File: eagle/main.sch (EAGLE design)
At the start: 43 parts, among them Q1 SQJ886EP, U1 LTC3789EGNPBF

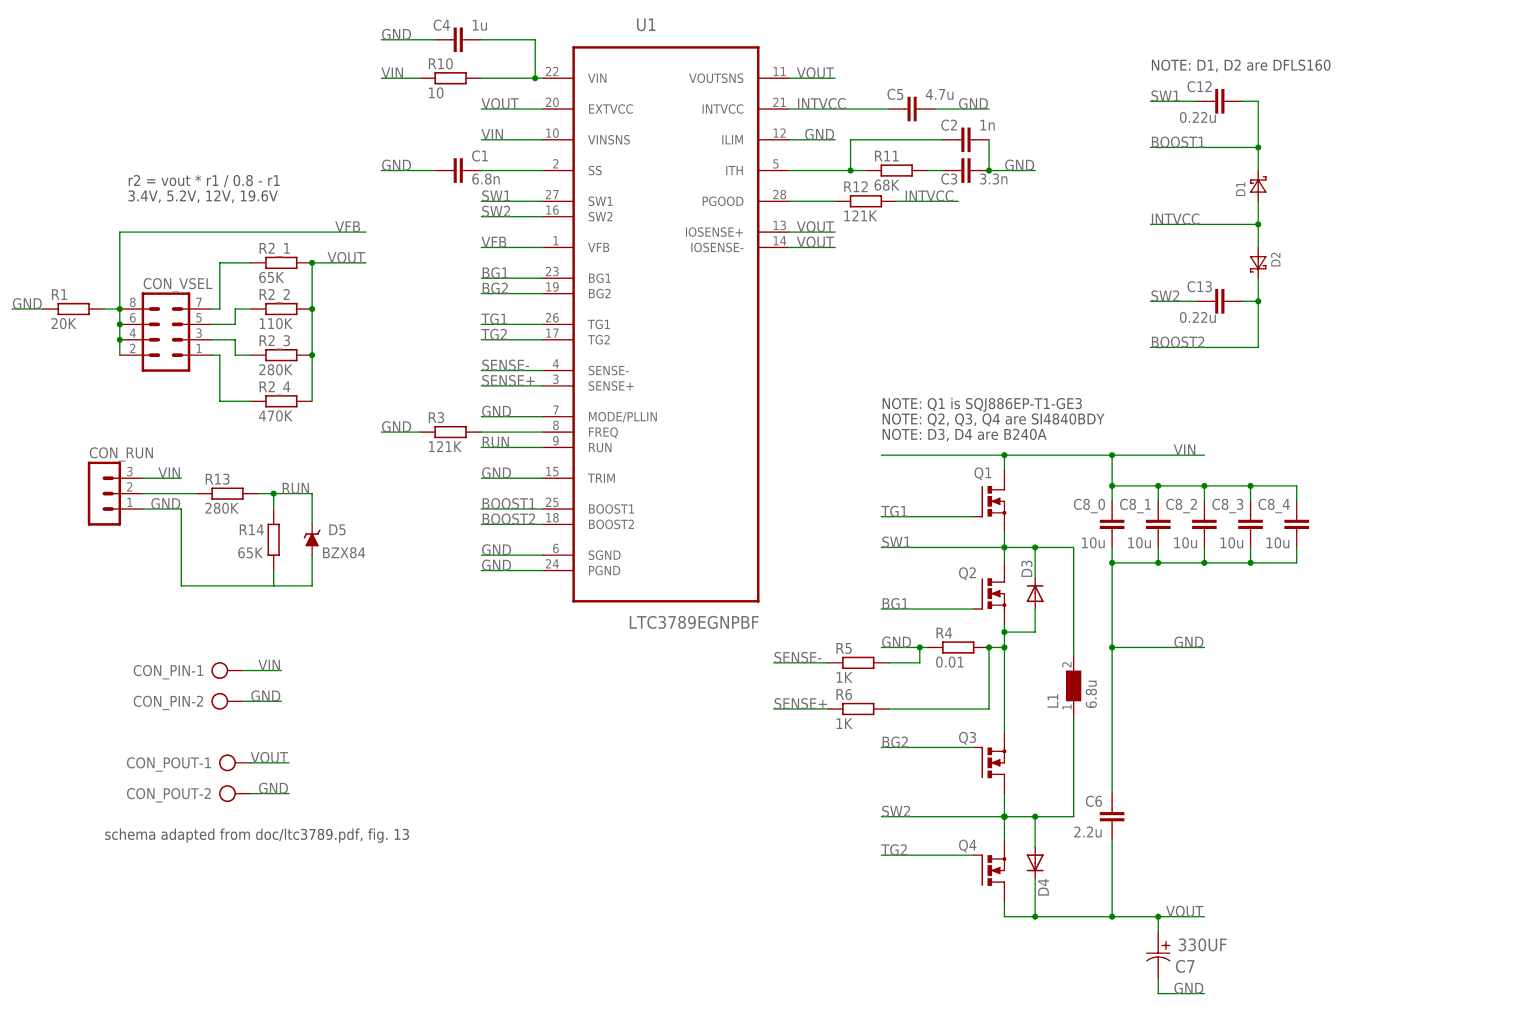
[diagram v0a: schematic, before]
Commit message: [ update ] sch
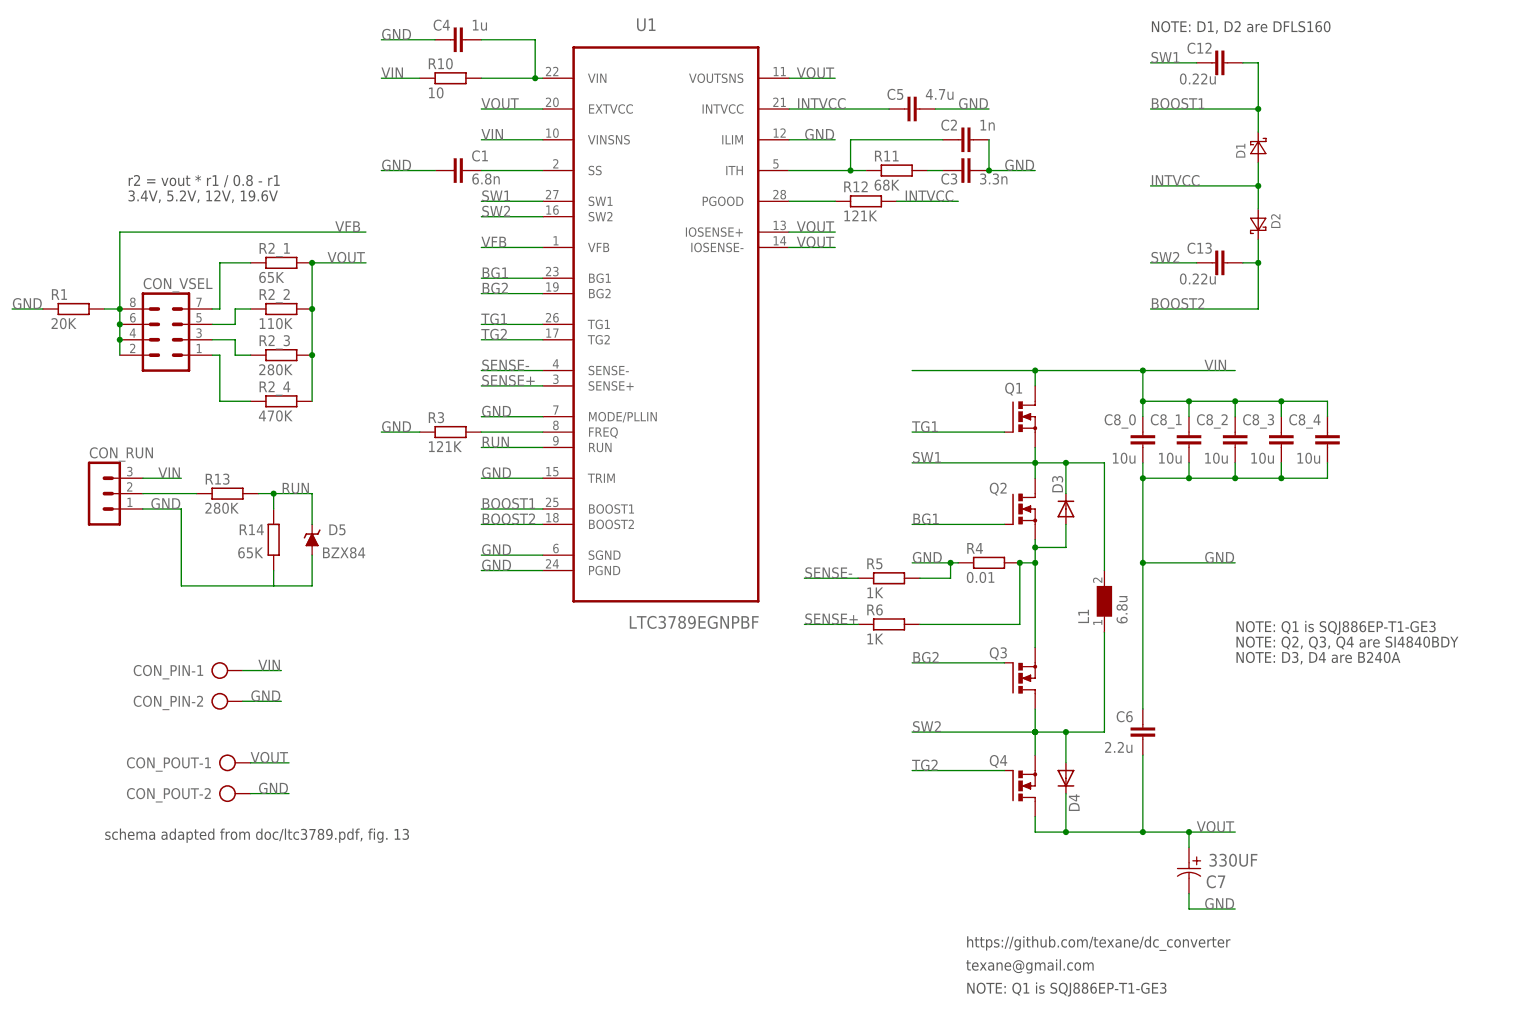
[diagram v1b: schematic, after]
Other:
- note added: "https://github.com/texane/dc_converter"
- note added: "texane@gmail.com"
- moved on the sheet: C12, C13, C6, C7, C8_0, C8_1, C8_2, C8_3, C8_4, D1, D2, D3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
